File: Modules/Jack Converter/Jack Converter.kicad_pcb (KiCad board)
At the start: 2 copper layers, 45 x 175 mm, 27 parts, among them J1 TS_Jack_3.5mm_Sw, J10 TS_Jack_6.35mm_Sw, J100 IDC_02x08, J11 TS_Jack_3.5mm_Sw, J12 TS_Jack_6.35mm_Sw, J13 TS_Jack_3.5mm_Sw, J14 TS_Jack_6.35mm_Sw, J15 TS_Jack_3.5mm_Sw, J16 TS_Jack_6.35mm_Sw, J17 TS_Jack_3.5mm_Sw, J18 TS_Jack_6.35mm_Sw, J2 TS_Jack_6.35mm_Sw, J3 TS_Jack_3.5mm_Sw, J4 TS_Jack_6.35mm_Sw, J5 TS_Jack_3.5mm_Sw, J50 Conn_01x08_BackboneTap, J6 TS_Jack_6.35mm_Sw, J7 TS_Jack_3.5mm_Sw, J8 TS_Jack_6.35mm_Sw, J9 TS_Jack_3.5mm_Sw, SW1 SW_DPDT, SW2 SW_DPDT, SW3 SW_DPDT

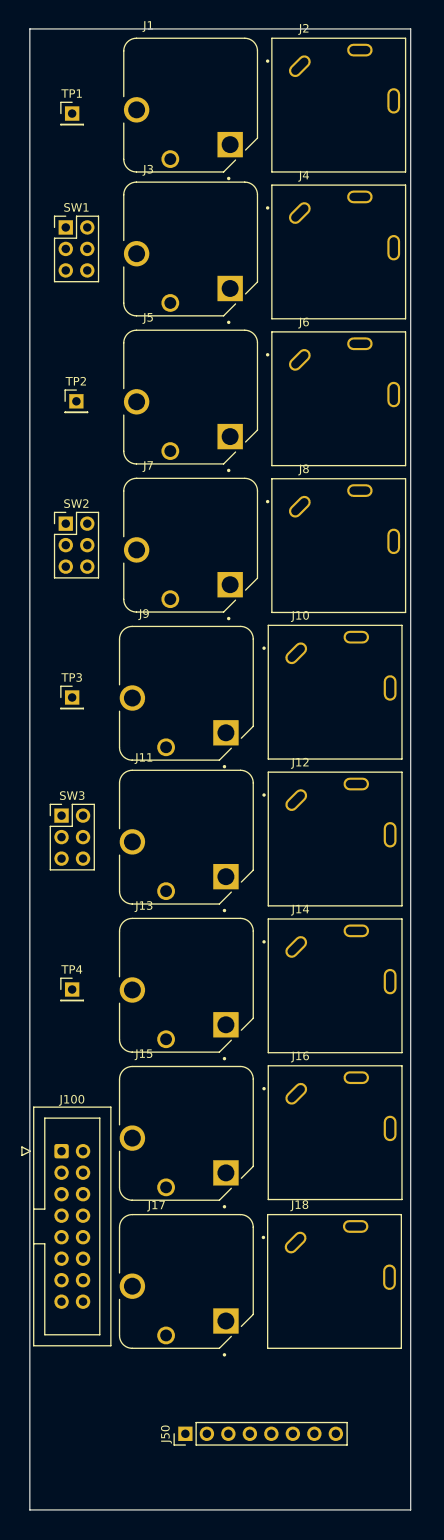
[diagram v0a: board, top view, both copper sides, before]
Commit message: Positioned components precisely
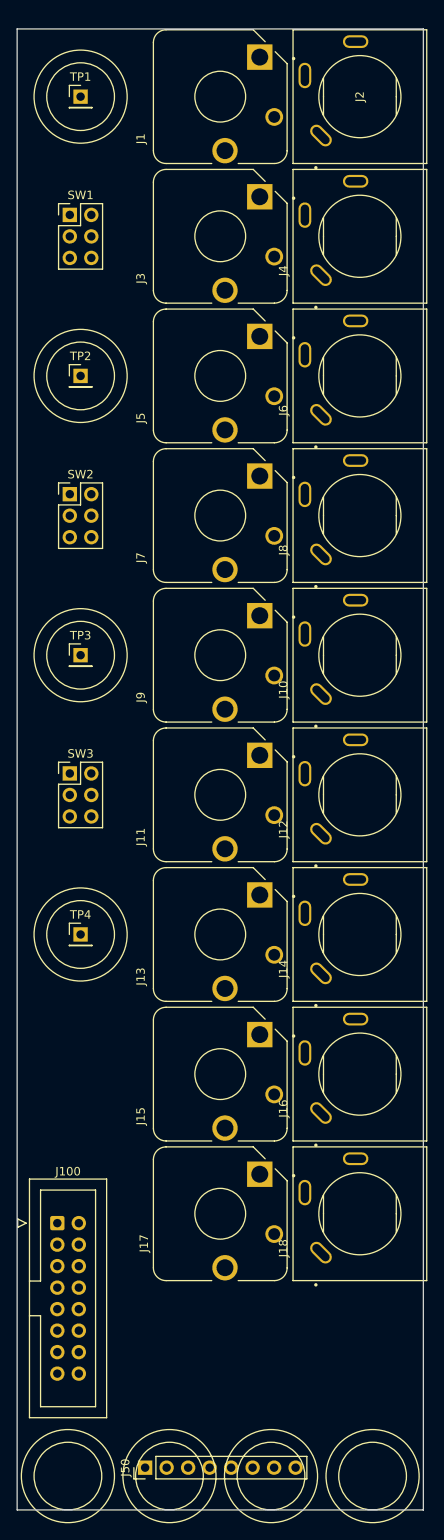
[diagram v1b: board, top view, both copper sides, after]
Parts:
- moved J17 8.94 mm to (72.5, 185.0), turned to 90 degrees
- moved J18 8.54 mm to (89.0, 185.0), turned to 90 degrees
- moved J100 8.51 mm to (53.2, 186.1)
- moved J15 8.06 mm to (72.5, 168.5), turned to 90 degrees
- moved J16 7.51 mm to (89.0, 168.5), turned to 90 degrees
- moved J13 7.21 mm to (72.5, 152.0), turned to 90 degrees
- moved J14 6.74 mm to (89.0, 152.0), turned to 90 degrees
- moved TP4 6.58 mm to (56.0, 152.0)
- moved J11 6.40 mm to (72.5, 135.5), turned to 90 degrees
- moved J50 6.21 mm to (63.6, 215.0)
- moved J9 6.02 mm to (72.5, 119.0), turned to 90 degrees
- moved J12 5.98 mm to (89.0, 135.5), turned to 90 degrees
- moved J10 5.26 mm to (89.0, 119.0), turned to 90 degrees
- moved TP3 5.10 mm to (56.0, 119.0)
- moved SW3 5.08 mm to (54.7, 133.0)
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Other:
- board size 45 x 175 mm -> 48 x 175 mm
